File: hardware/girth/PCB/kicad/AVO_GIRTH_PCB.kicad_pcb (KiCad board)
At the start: 4 copper layers, 65.5 x 43.5 mm, 122 parts, among them J1 USB-C 16P, J2 BATERÍA 1S, K1 G6KU-2F-Y DC3, Q1 AO3401A, Q10 AO3401A, Q11 AO3400A, Q12 2N7002, Q13 AO3400A, Q14 AO3401A, Q15 2N7002, Q16 2N7002, Q17 AO3401A, Q18 2N7002, Q2 AO3401A, Q3 AO3401A, SW1 REED (1), SW2 REED (2), U1 BQ51013BRHLR, U2 BQ24072RGTR, U3 RT9080-33GJ5, U4 ESP32-C6-MINI-1U-N4, U5 BNO085, U6 USBLC6-2SC6, Y1 32,768 kHz 12,5 pF

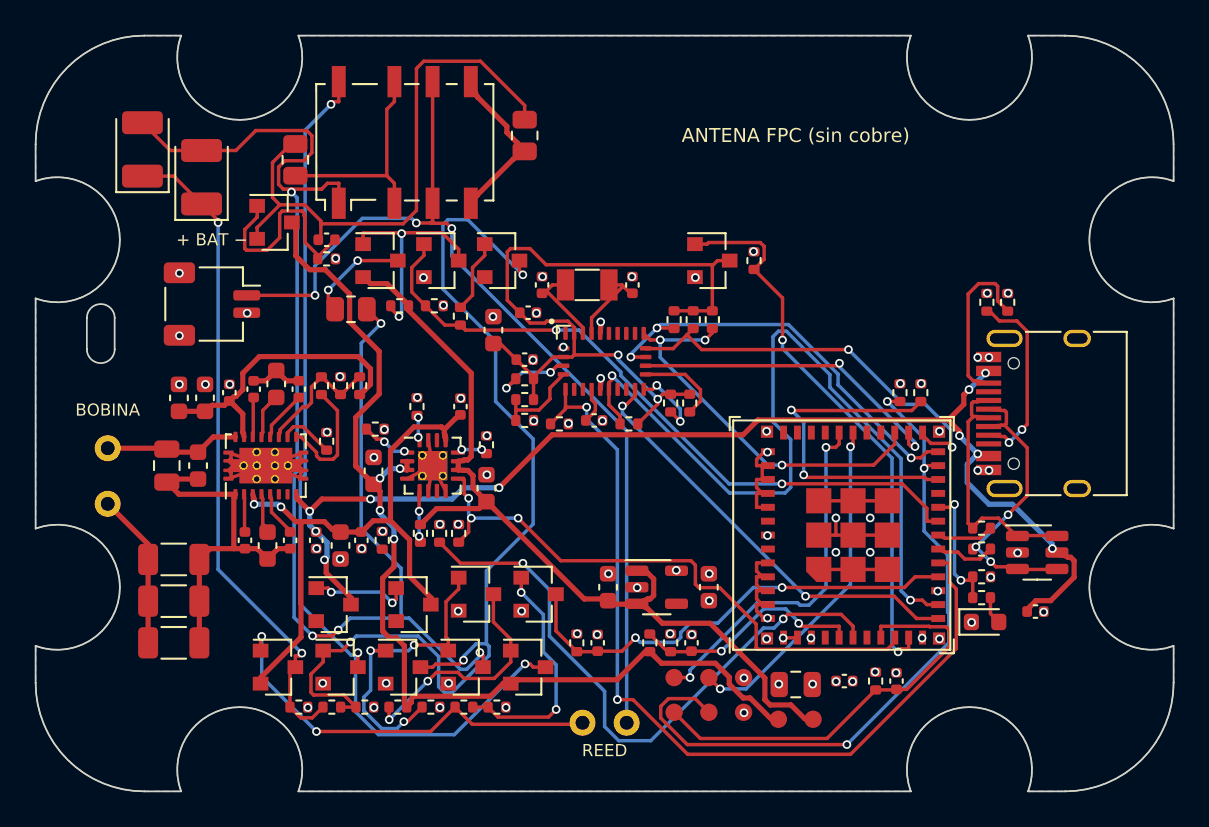
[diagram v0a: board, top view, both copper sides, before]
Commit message: PCB cincha: resultados de KiCad 9 de 8f7eaff (puerta: false) [skip ci]
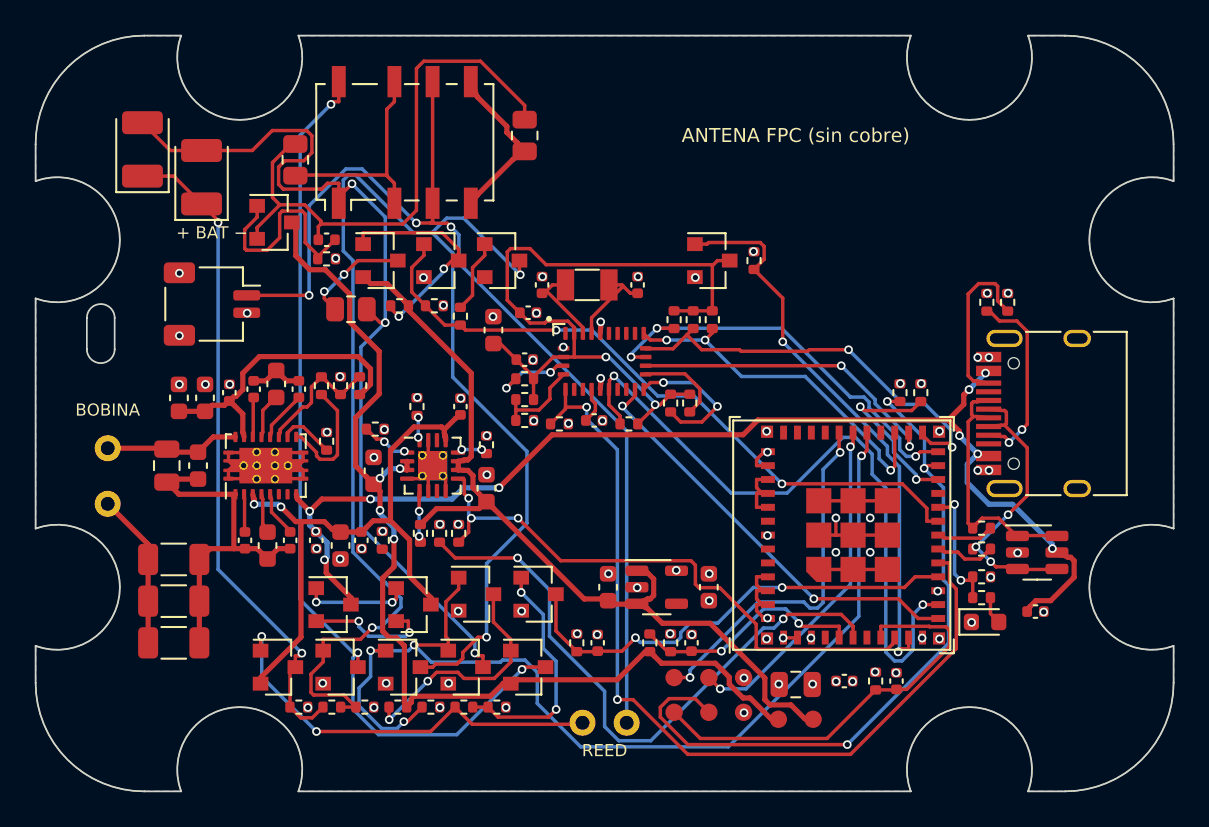
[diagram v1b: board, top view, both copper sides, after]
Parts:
- moved C28 0.30 mm to (101.9, 92.6)
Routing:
- net RLY_OFF: track 17.9 -> 61.2 mm, vias 3 -> 4
- net RLY_GB: track 59.2 -> 83.9 mm
- net K_A: track 78.7 -> 54.8 mm, vias 5 -> 3
- net GPIO8: track 19.6 -> 10.6 mm
- net AD_SRC: track 0.00 -> 7.39 mm, vias 0 -> 2
- net IMU_RST: track 46.5 -> 40.0 mm
- net BAT_RAW: track 55.7 -> 60.1 mm
- net IMU_ENV_SCL: track 4.27 -> 8.28 mm
- net GND: track 45.7 -> 42.7 mm
- net IMU_MISO: track 22.8 -> 20.9 mm
- net IMU_MOSI: track 18.9 -> 18.4 mm
